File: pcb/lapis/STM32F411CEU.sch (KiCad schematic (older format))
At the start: 11 parts, among them IC5 STM32G484CET6, U1 STM32F411CEUx

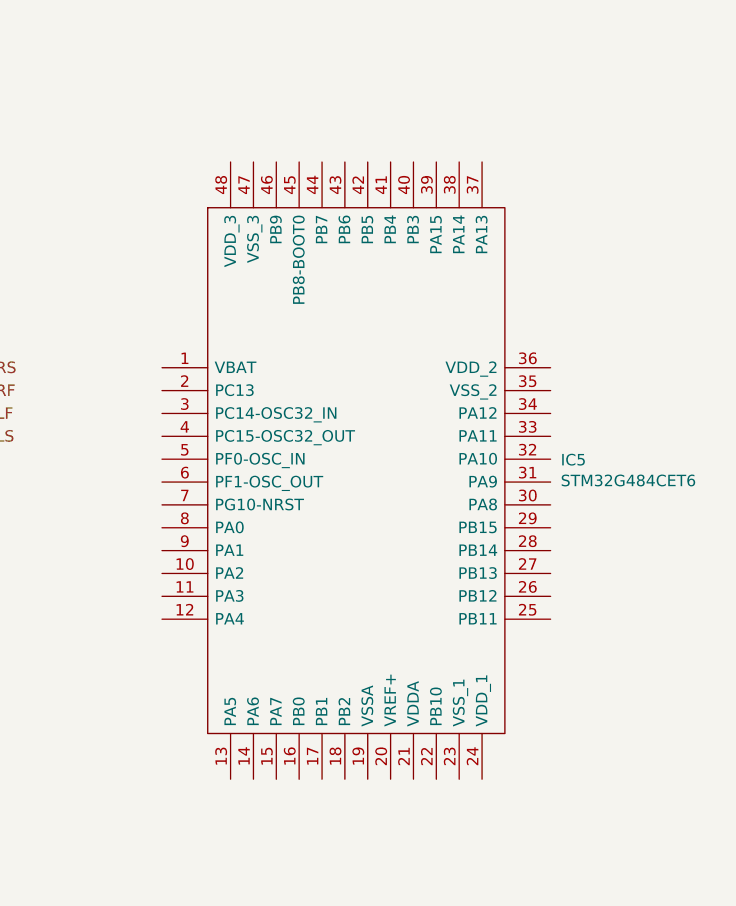
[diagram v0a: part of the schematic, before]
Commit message: no message
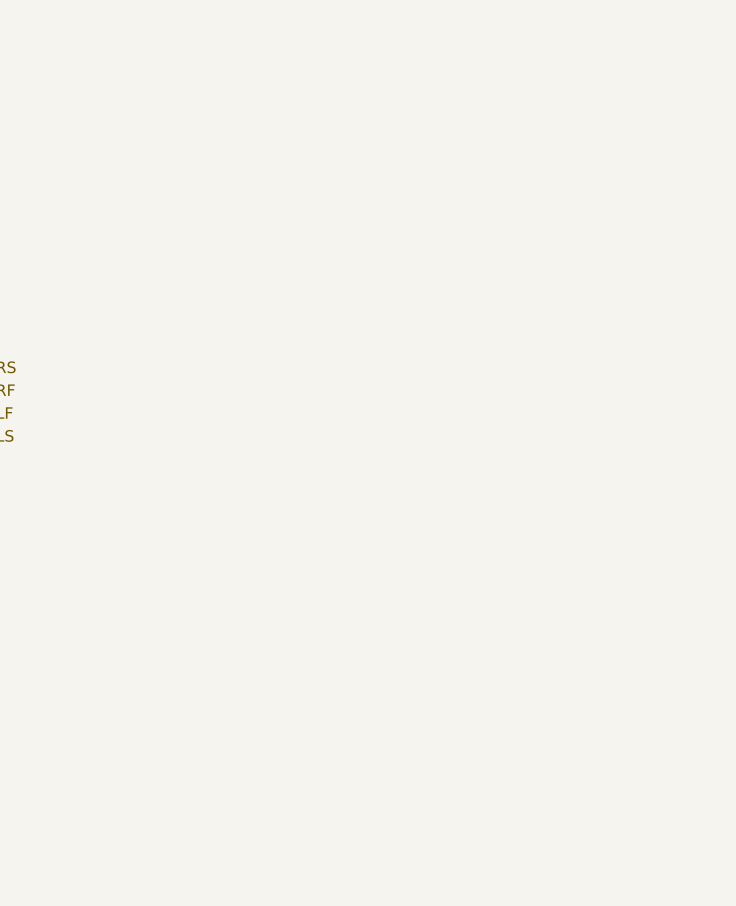
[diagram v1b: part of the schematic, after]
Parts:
- removed IC5: STM32G484CET6, Package_QFP:LQFP-48_7x7mm_P0.5mm, symbol SamacSys_Parts:STM32G484CET6
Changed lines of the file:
@@
 Text HLabel 7950 5200 2    50   Output ~ 0
 SPEAKER
-$Comp
-L SamacSys_Parts:STM32G484CET6 IC5
-U 1 1 618978F9
-P 9250 3700
-F 0 "IC5" H 10994 3296 50  0000 L CNN
-F 1 "STM32G484CET6" H 10994 3205 50  0000 L CNN
-F 2 "Package_QFP:LQFP-48_7x7mm_P0.5mm" H 10800 4400 50  0001 L CNN
-F 3 "" H 10800 4300 50  0001 L CNN
-F 4 "MCU, 32BIT, 170MHZ, LQFP-48" H 10800 4200 50  0001 L CNN "Description"
-F 5 "1.6" H 10800 4100 50  0001 L CNN "Height"
-F 6 "" H 10800 4000 50  0001 L CNN "RS Part Number"
-F 7 "" H 10800 3900 50  0001 L CNN "RS Price/Stock"
-F 8 "STMicroelectronics" H 10800 3800 50  0001 L CNN "Manufacturer_Name"
-F 9 "STM32G484CET6" H 10800 3700 50  0001 L CNN "Manufacturer_Part_Number"
-	1    9250 3700
-	1    0    0    -1
-$EndComp
 $EndSCHEMATC
